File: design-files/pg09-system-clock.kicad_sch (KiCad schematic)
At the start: 15 parts, among them J201 Clock Speed, Q201 2N7000, U201 CD74ACT109, U202 CD74ACT163, U204 GAL22V10, X201 ACO-32.000MHz

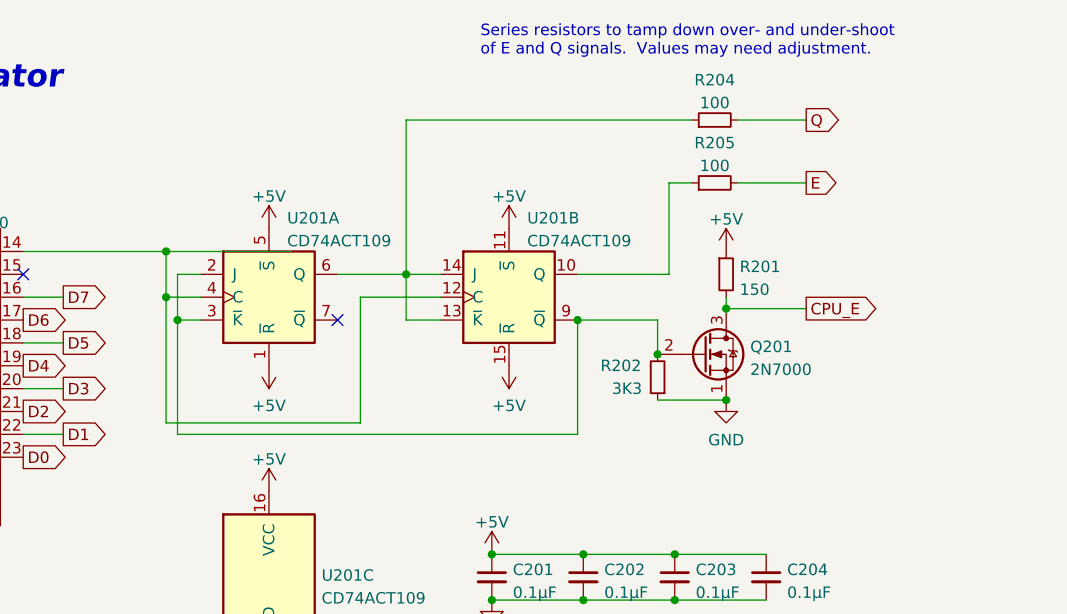
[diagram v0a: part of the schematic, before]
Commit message: Remove CPU_E and the associated circuitry -- measurements on a prototype indicate that it's not necessary.
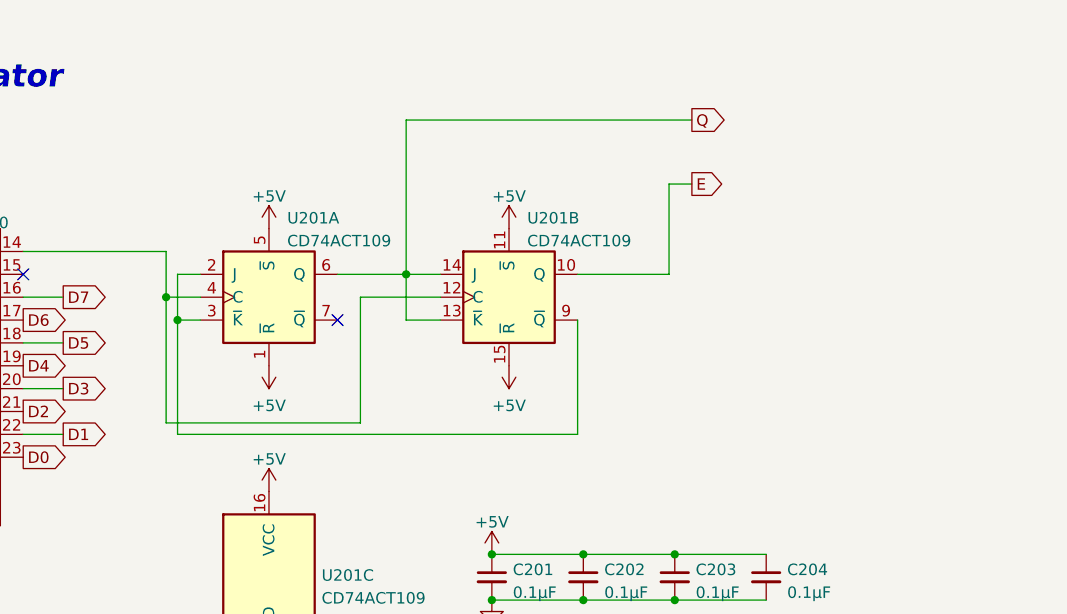
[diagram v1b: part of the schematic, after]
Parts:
- removed Q201: 2N7000, Package_TO_SOT_THT:TO-92_Inline, symbol Transistor_FET:2N7000
- removed R201: 150, Resistor_THT:R_Axial_DIN0207_L6.3mm_D2.5mm_P7.62mm_Horizontal, symbol Device:R_Small
- removed R202: 3K3, Resistor_THT:R_Axial_DIN0207_L6.3mm_D2.5mm_P7.62mm_Horizontal, symbol Device:R_Small
- removed R204, R205: 100, Resistor_THT:R_Axial_DIN0207_L6.3mm_D2.5mm_P7.62mm_Horizontal, symbol Device:R_Small
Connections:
- net E: now also U201.10 (Q)
- net Q: now also U201.13 (~{K}), U201.14 (J), U201.6 (Q)
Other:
- note removed: "Series resistors to tamp down over- and under-shoot of E and Q signals. Values may need adjustment."
